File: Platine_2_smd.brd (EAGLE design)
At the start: 88.9 x 101.6 mm, 19 parts, among them X2 DTF13-12PA

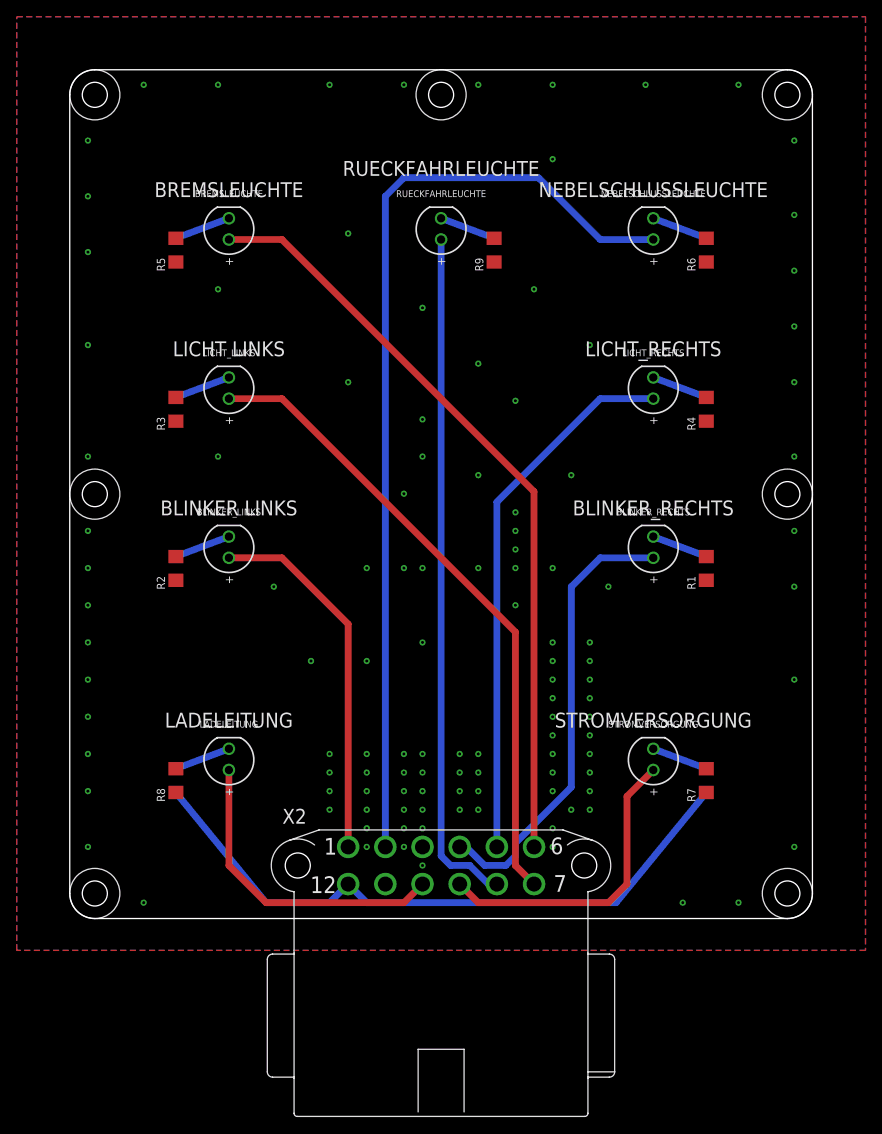
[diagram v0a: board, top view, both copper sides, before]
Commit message: Done !
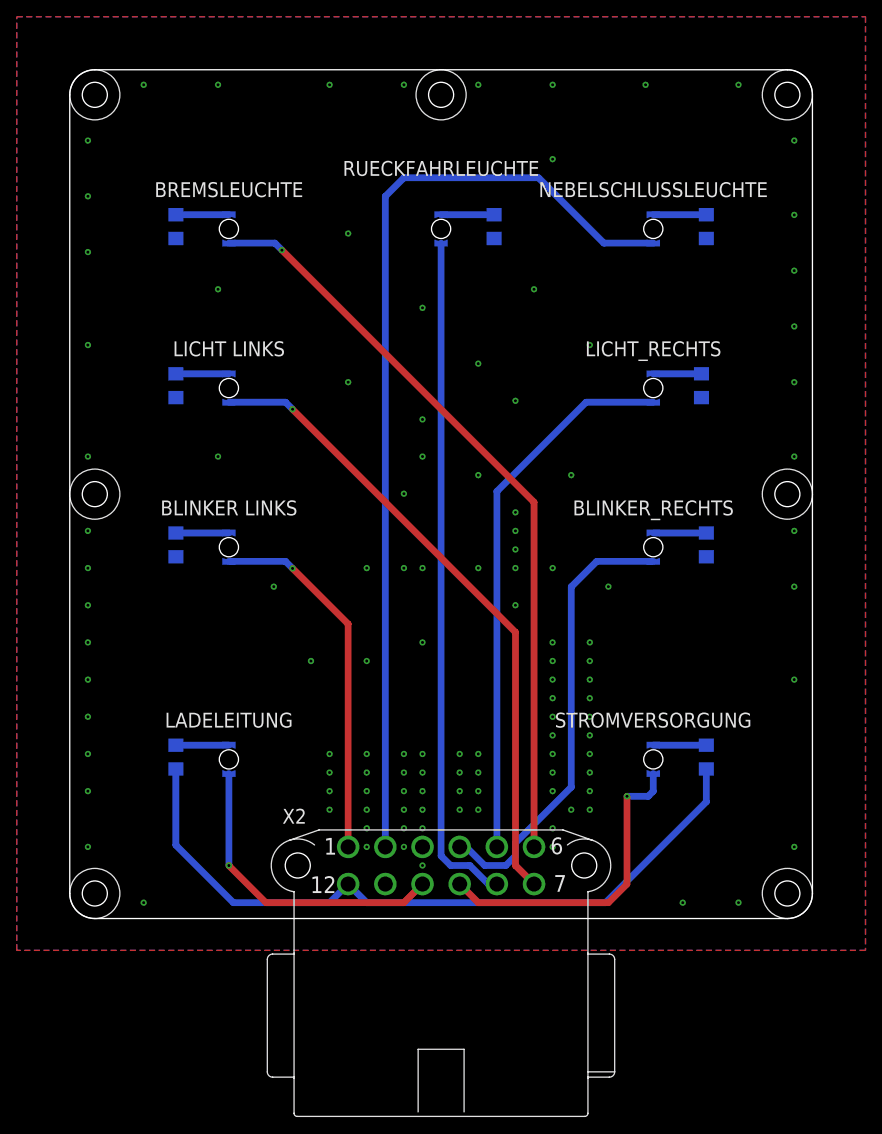
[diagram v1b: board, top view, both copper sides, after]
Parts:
- BLINKER_LINKS, BLINKER_RECHTS, BREMSLEUCHTE, LADELEITUNG, LICHT_LINKS, LICHT_RECHTS, NEBELSCHLUSSLEUCHTE, RUECKFAHRLEUCHTE, STROMVERSORGUNG: device Wurth_LEDs_WL-TMRW:WL-TMRW_5MM -> Wurth_LEDs_WL-SMRW:WL-SMRW_1206_DOME_REV
- moved R4 2.88 mm to (31.2, 57.4), flipped to the bottom
- moved R7 2.82 mm to (31.8, 13.0), flipped to the bottom
- moved R8 2.82 mm to (-31.8, 13.0), flipped to the bottom
- moved R1 2.82 mm to (31.8, 38.4), flipped to the bottom
- moved R2 2.82 mm to (-31.8, 38.4), flipped to the bottom
- moved R3 2.82 mm to (-31.8, 57.4), flipped to the bottom
- moved R5 2.82 mm to (-31.8, 76.5), flipped to the bottom
- moved R6 2.82 mm to (31.8, 76.5), flipped to the bottom
- moved R9 2.82 mm to (6.35, 76.5), flipped to the bottom
- flipped BLINKER_LINKS to the bottom, turned to 270 degrees
- flipped BLINKER_RECHTS to the bottom, turned to 270 degrees
- flipped BREMSLEUCHTE to the bottom, turned to 270 degrees
- flipped LADELEITUNG to the bottom, turned to 270 degrees
- flipped LICHT_LINKS to the bottom, turned to 270 degrees
- flipped LICHT_RECHTS to the bottom, turned to 270 degrees
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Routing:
- net MASSE_9: track 77.8 -> 86.3 mm
- net STROMVERSORGUNG_9: track 36.8 -> 37.9 mm, vias 0 -> 1
- net N$2: track 6.78 -> 5.77 mm
- net BREMSLEUCHTE_6: track 91.6 -> 90.6 mm, vias 0 -> 1
- net LICHT_RECHTS_5: track 65.1 -> 65.7 mm
- net LADELEITUNG_10: track 37.4 -> 36.9 mm, vias 0 -> 1
- net BLINKER_LINKS_1: track 44.2 -> 44.1 mm, vias 0 -> 1
- net LICHT_LINKS_7: track 77.0 -> 76.8 mm, vias 0 -> 1
